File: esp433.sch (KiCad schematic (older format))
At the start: 35 parts, among them J1 USB_OTG, J2 CONN_01X03, Q1 MBT2222ADW1T1, SW1 SW_Push, U1 AP2127K-3.3, U2 IRM-02-5, U3 ESP-12E, U4 FT231XS

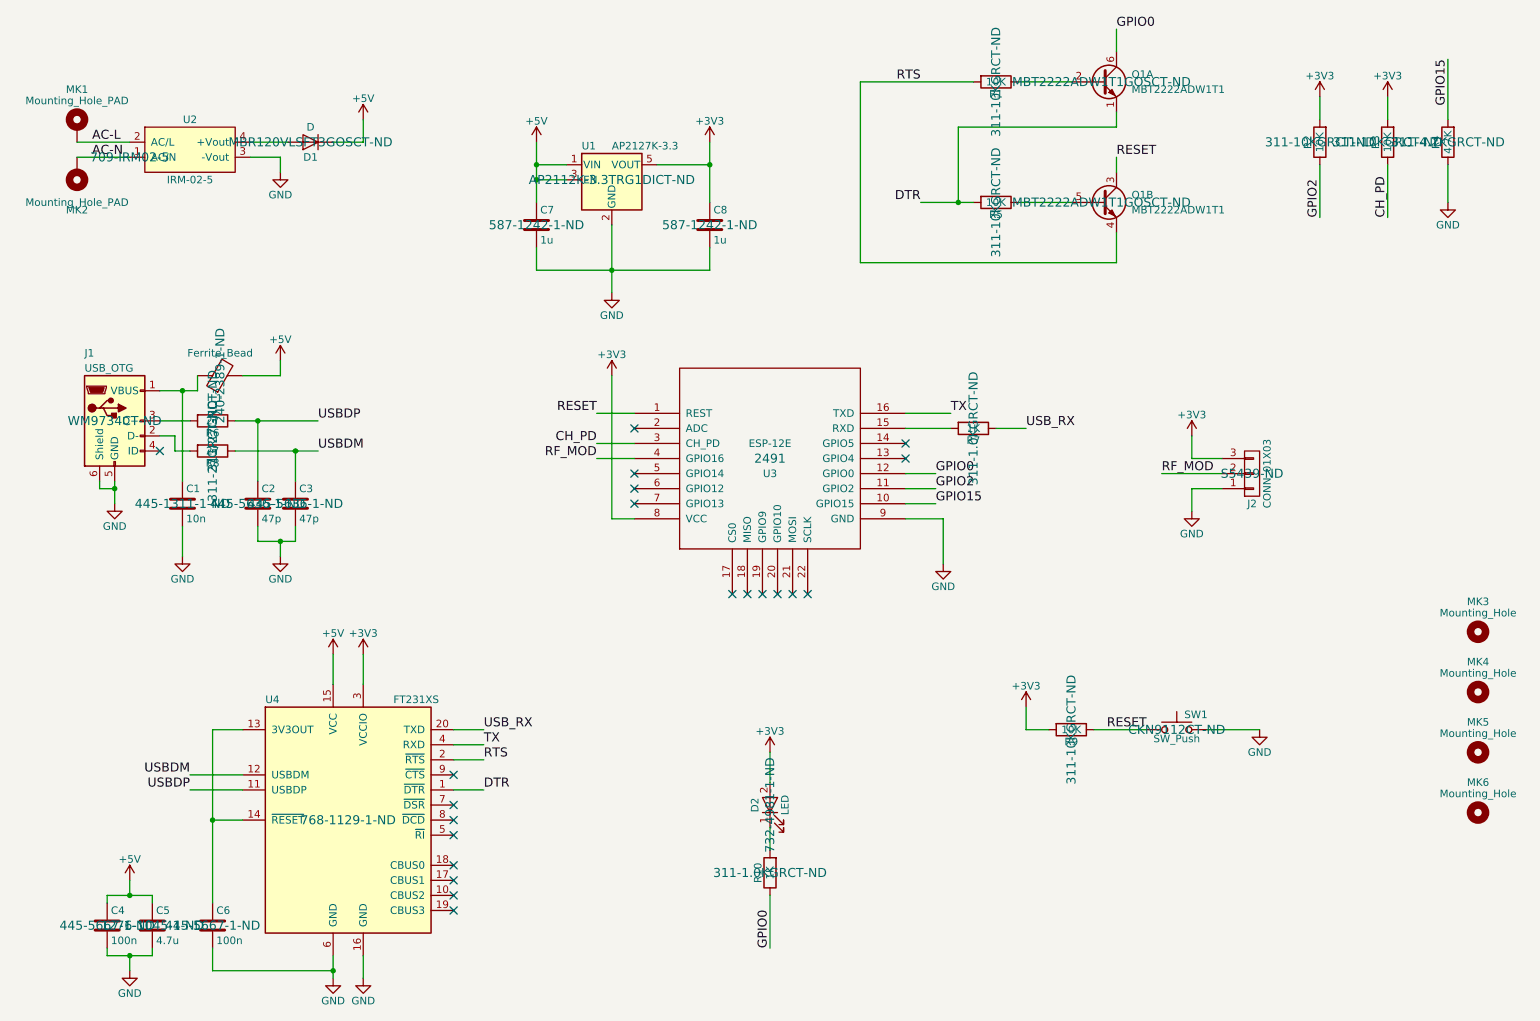
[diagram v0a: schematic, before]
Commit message: Add rf circuit
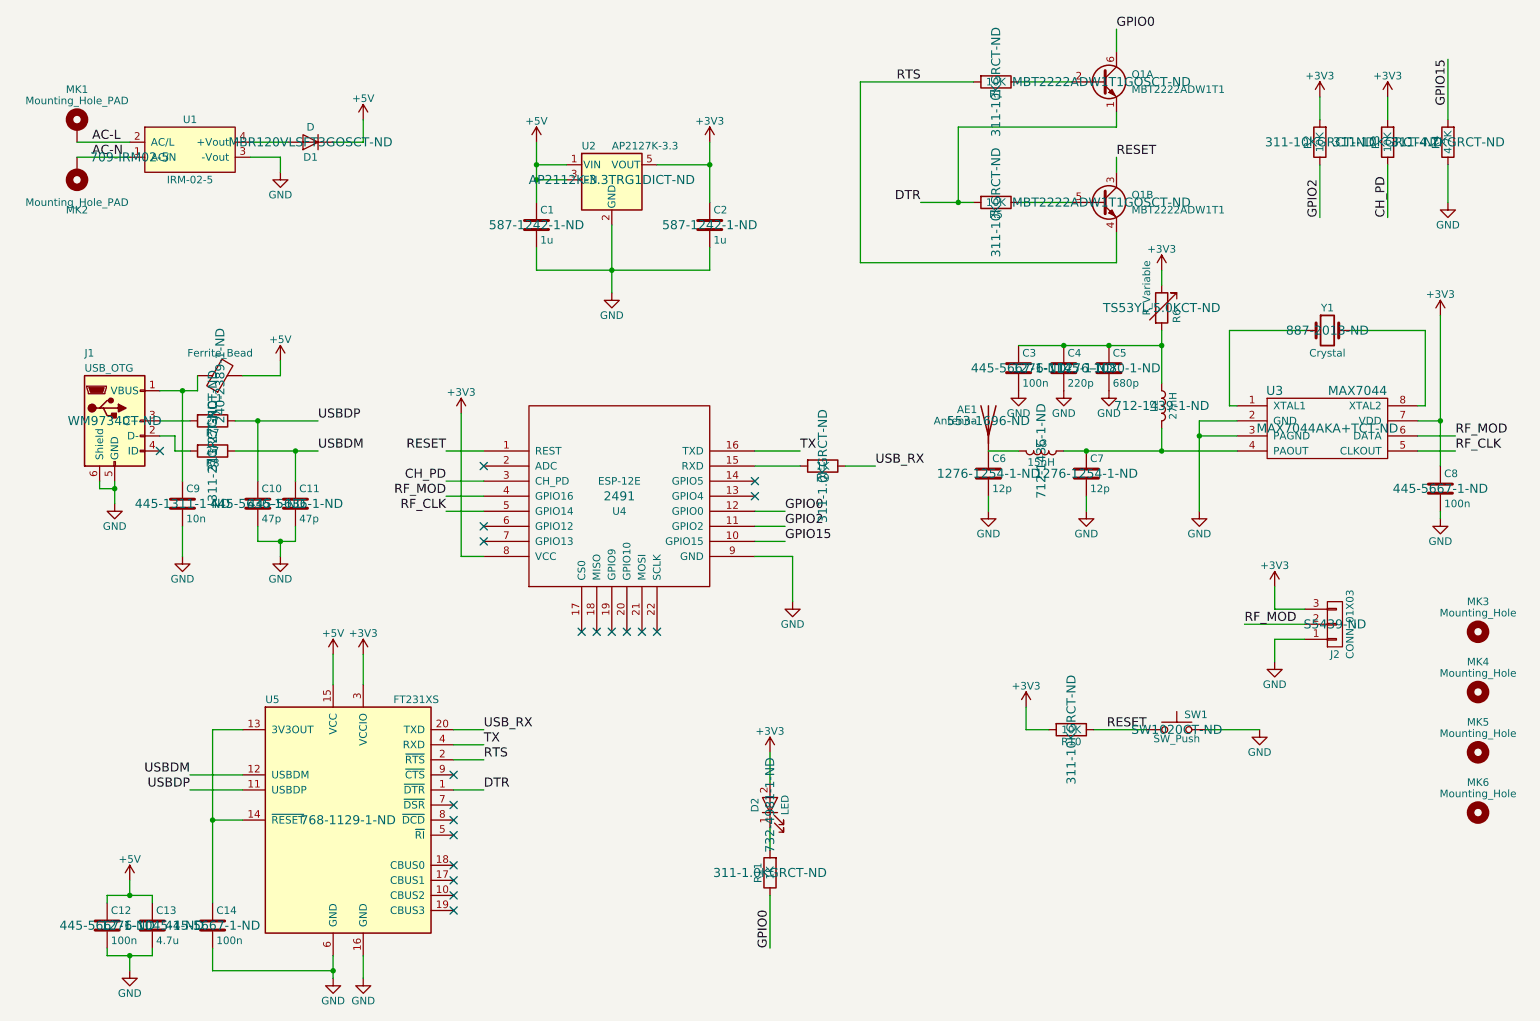
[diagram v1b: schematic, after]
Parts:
- added AE1: Antenna, esp433:W3127, symbol Antenna
- added C3, C8: 100n, Capacitors_SMD:C_0603, symbol C
- added C4: 220p, Capacitors_SMD:C_0603, symbol C
- added C5: 680p, Capacitors_SMD:C_0603, symbol C
- added C6, C7: 12p, Capacitors_SMD:C_0603, symbol C
- added L2: 27nH, Inductors_SMD:L_0603, symbol L
- added L3: 15nH, Inductors_SMD:L_0603, symbol L
- added R6: R_Variable, Potentiometers:Potentiometer_Trimmer_Vishay_TS53YL, symbol R_Variable
- added U3: MAX7044, TO_SOT_Packages_SMD:SOT-23-8, symbol MAX7044
- added Y1: Crystal, Crystals:Crystal_HC49-U_Vertical, symbol Crystal
- SW1: footprint Buttons_Switches_SMD:SW_SPST_PTS645 -> Buttons_Switches_SMD:SW_SPST_B3U-1000P; Vendorpart CKN9112CT-ND -> SW1020CT-ND
- renumbered C7 to C1, C2 to C10, C3 to C11, C4 to C12, C5 to C13, C6 to C14, C8 to C2, C1 to C9, R9 to R10, R10 to R11, R6 to R7, R7 to R9, U2 to U1, U1 to U2, U3 to U4, U4 to U5
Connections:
- net +3V3: now also C8.1, R6.1, U3.7 (VDD)
- net GND: now also C3.2, C4.2, C5.2, C6.2, C7.2, C8.2, U3.2 (GND), U3.3 (PAGND)
- net RF_MOD: now also U3.6 (DATA)
- net RF_CLK: now reaches U4.5 (GPIO14)
- net RF_CLK: now also U3.5 (CLKOUT)
- new net: U3.1 (XTAL1), Y1.1
- new net: C7.1, L2.2, L3.1, U3.4 (PAOUT)
- new net: U3.8 (XTAL2), Y1.2
- new net: C3.1, C4.1, C5.1, L2.1, R6.2
- new net: AE1.1 (A), C6.1, L3.2
- no-connect marks 21 -> 20
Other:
- moved on the sheet: J2, R9, U4
